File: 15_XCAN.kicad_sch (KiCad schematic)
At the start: 5 parts, among them J1 Conn_01x06, J7 Conn_01x01, U1 MCP2551-I-SN

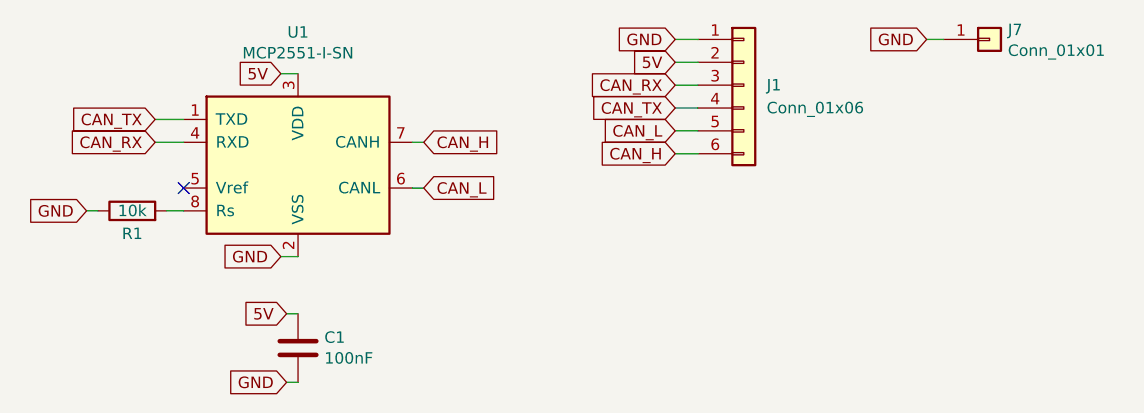
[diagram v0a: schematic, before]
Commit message: maj fichiers de fabrication
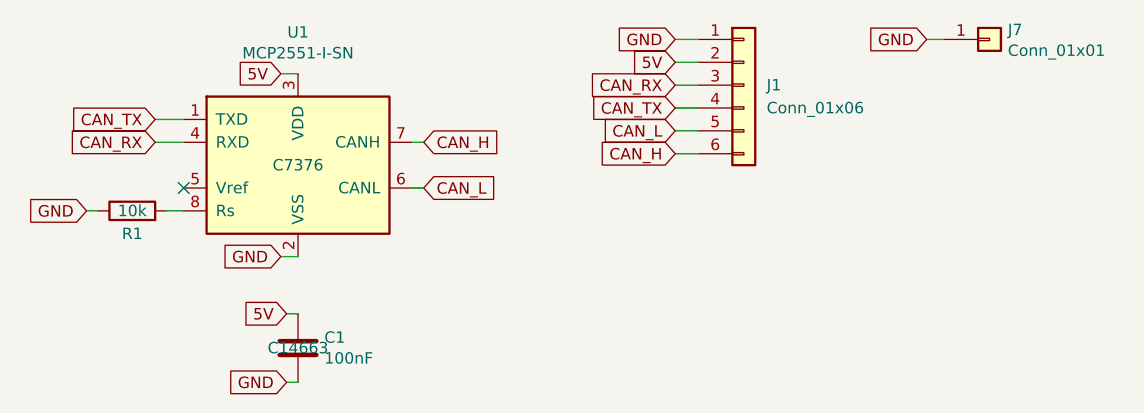
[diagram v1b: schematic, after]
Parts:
- C1: LCSC (none) -> C14663
- U1: LCSC (none) -> C7376
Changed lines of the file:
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@@
       (effects (font (size 1.27 1.27) italic) hide)
     )
-    (property "Datasheet" "C7376" (id 3) (at 63.5 46.99 0)
+    (property "Datasheet" "-" (id 3) (at 63.5 46.99 0)
       (effects (font (size 1.27 1.27)) hide)
     )
+    (property "LCSC" "C7376" (id 4) (at 63.5 46.99 0))
     (pin "1")
     (pin "2")
@@
       (effects (font (size 1.27 1.27)) hide)
     )
-    (property "Datasheet" "C14663" (id 3) (at 63.5 67.31 0)
+    (property "Datasheet" "-" (id 3) (at 63.5 67.31 0)
       (effects (font (size 1.27 1.27)) hide)
     )
+    (property "LCSC" "C14663" (id 4) (at 63.5 67.31 0))
     (pin "1")
     (pin "2")
